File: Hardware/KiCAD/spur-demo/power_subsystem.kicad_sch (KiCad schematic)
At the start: 29 parts, among them IC1 BQ24193RGER, IC3 ISL91127IRNZ-T7A, J5 Screw_Terminal_01x02, Q1 IRLZ44N

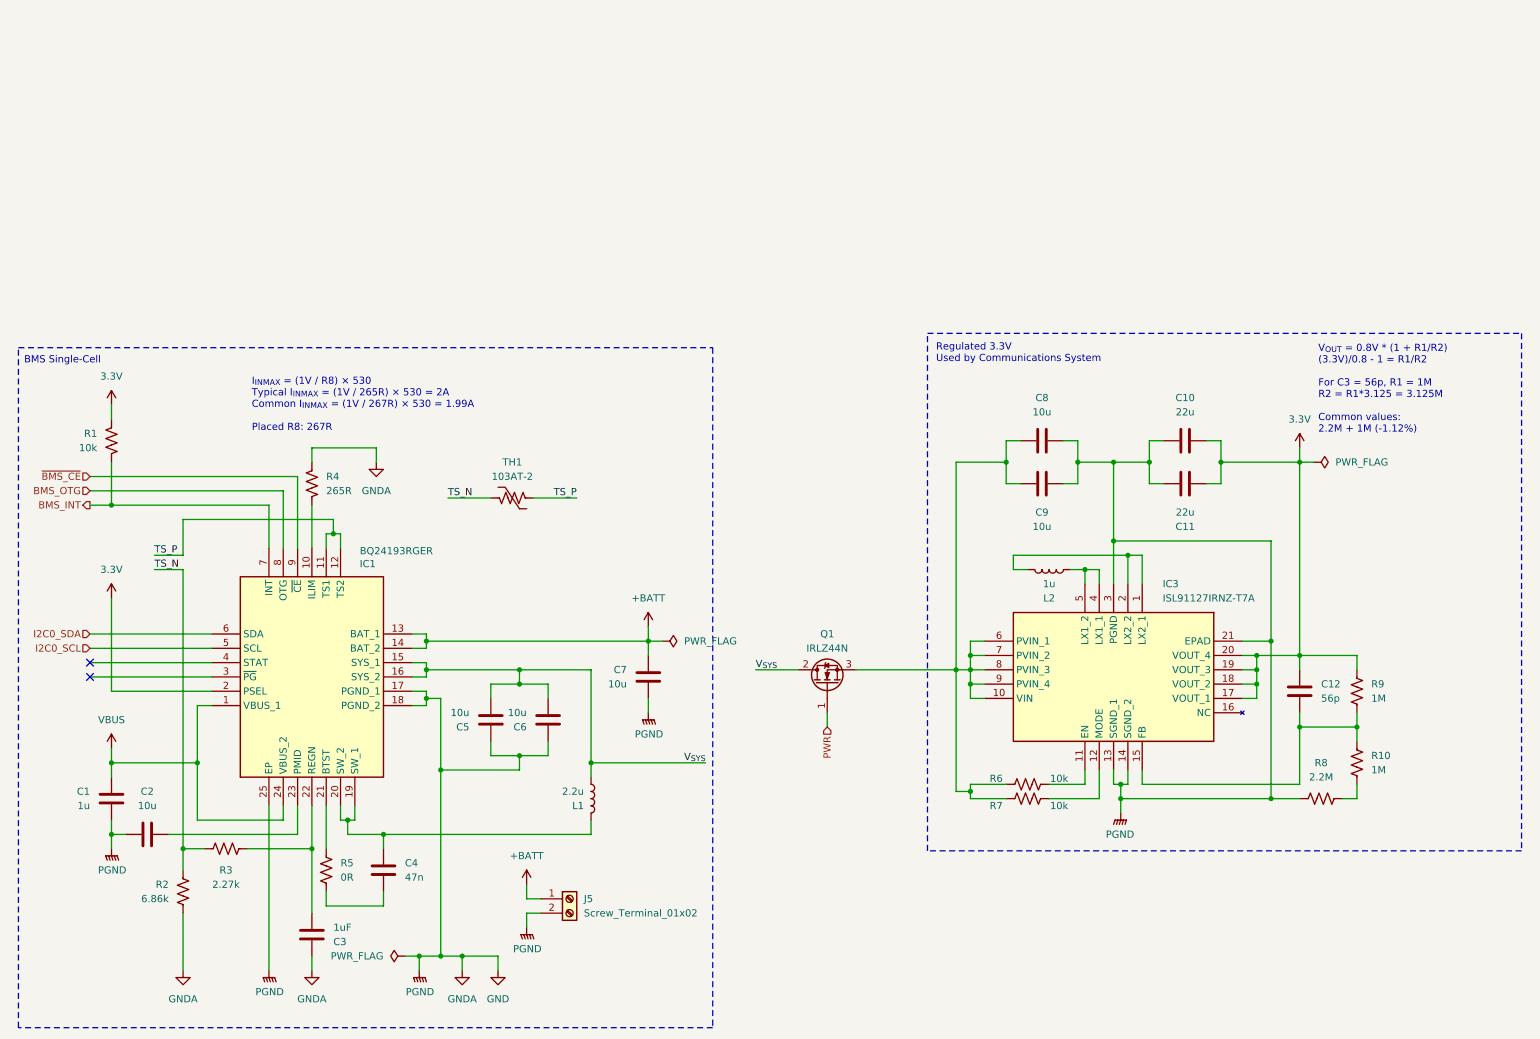
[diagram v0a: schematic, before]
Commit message: feat: add stat & pg indicators, psel solder jumper, begin power switch
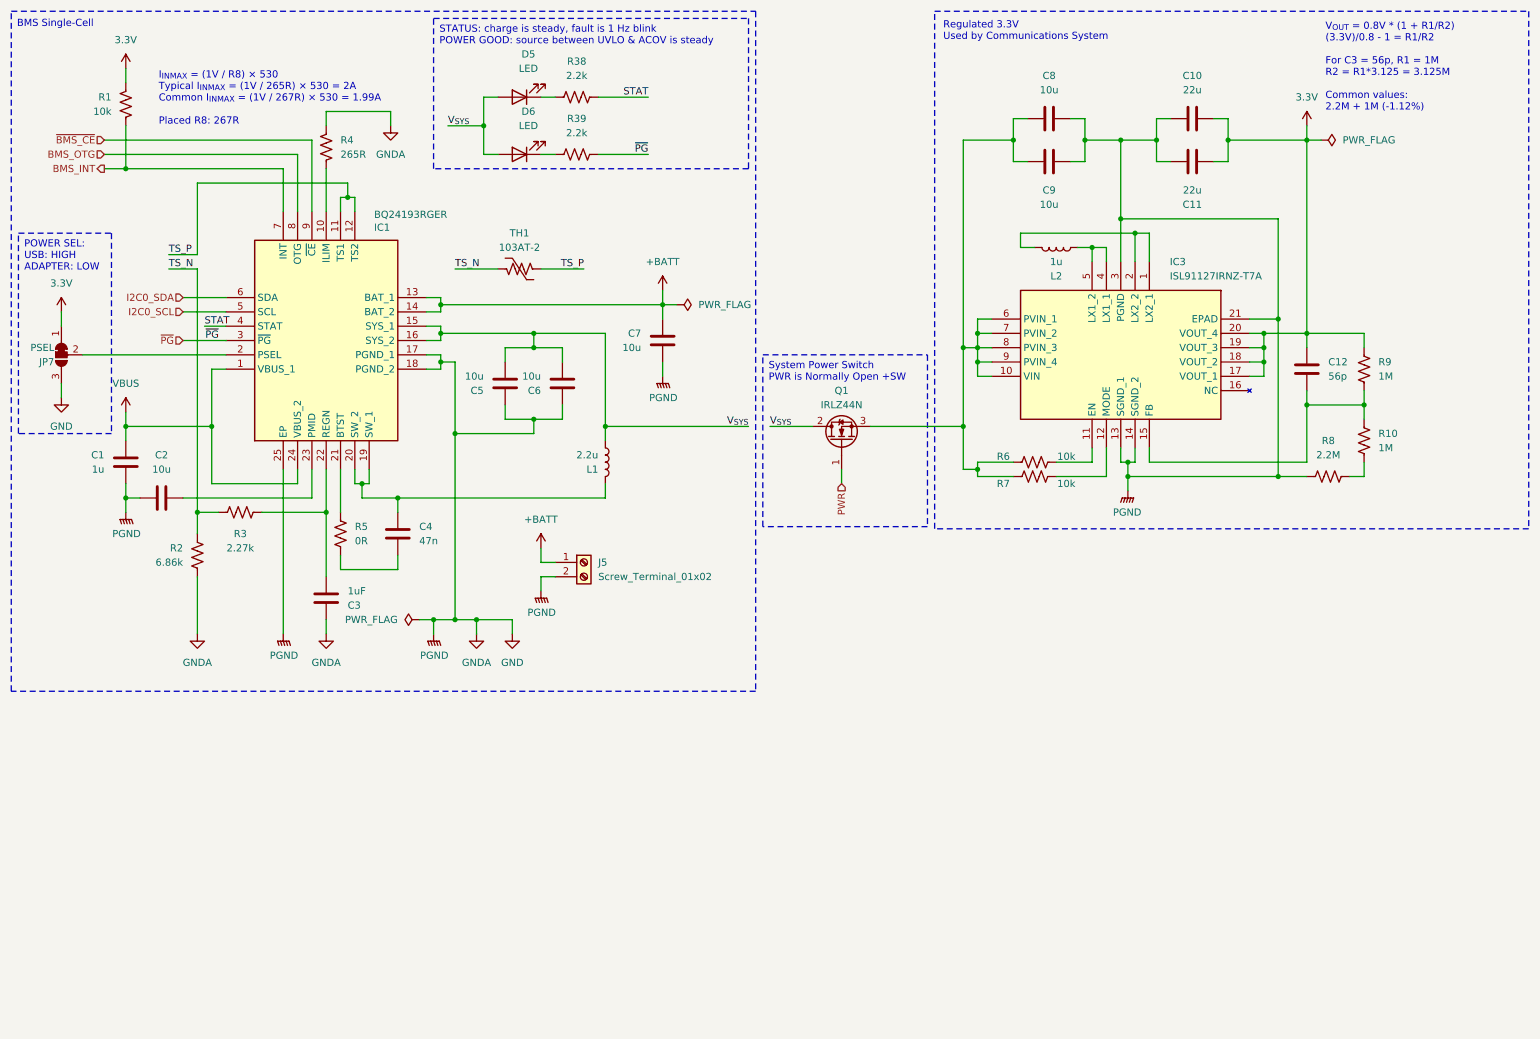
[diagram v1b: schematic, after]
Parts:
- added D5, D6: LED, symbol Device:LED
- added JP7: PSEL, symbol Jumper:SolderJumper_3_Bridged12
- added R38, R39: 2.2k, symbol Device:R_US
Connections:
- net 3.3V: now also JP7.1 (A); no longer IC1.2 (PSEL)
- net GND: now also JP7.3 (B)
- net V_{SYS}: now also D5.2 (A), D6.2 (A)
- net ~{PG}: now reaches IC1.3 (~{PG})
- net ~{PG}: now also R39.2
- net STAT: now reaches IC1.4 (STAT)
- net STAT: now also R38.2
- new net: D6.1 (K), R39.1
- new net: D5.1 (K), R38.1
- new net: IC1.2 (PSEL), JP7.2 (C)
- no-connect marks 2 -> 0
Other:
- moved on the sheet: C1, C10, C11, C12, C2, C3, C4, C5, C6, C7, C8, C9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
